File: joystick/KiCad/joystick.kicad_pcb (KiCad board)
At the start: 2 copper layers, 37 x 33 mm, 7 parts, among them J1 Conn_01x06_Pin, U1 COM-09032

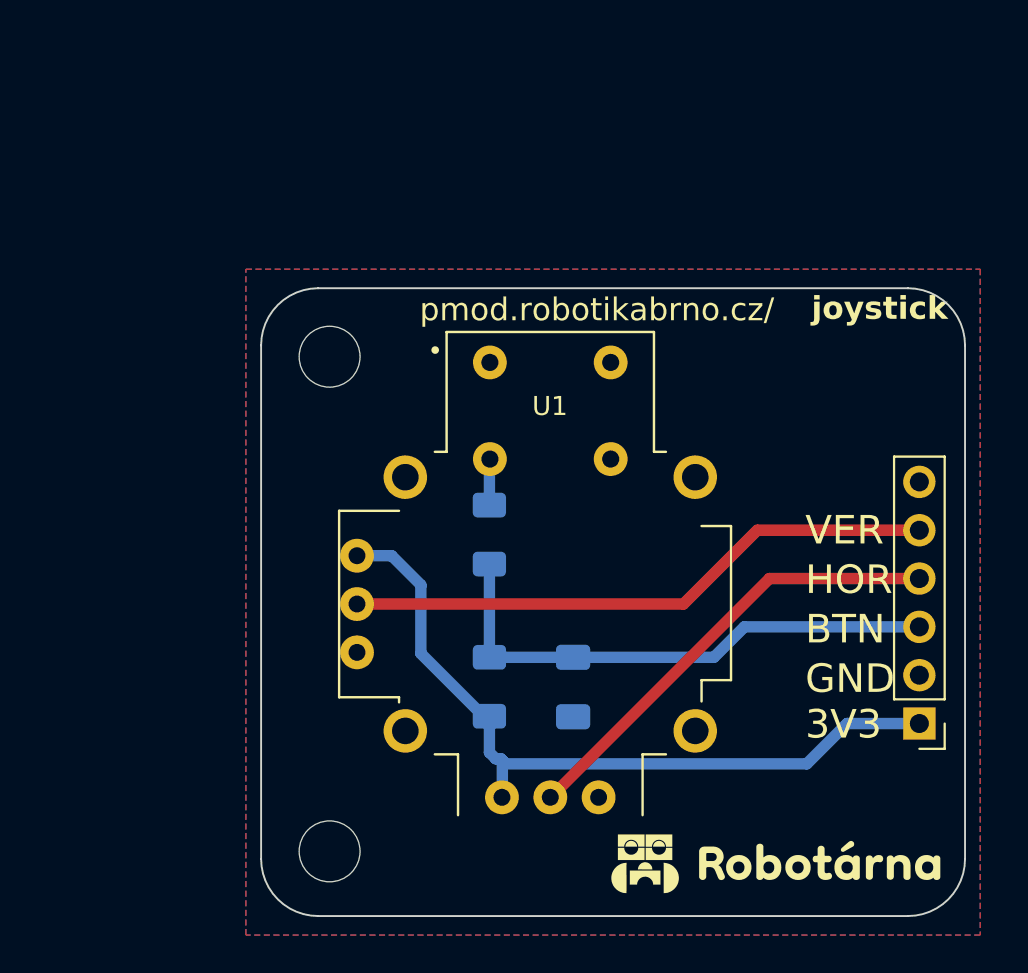
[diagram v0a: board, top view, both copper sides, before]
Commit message: Deployed d972a79 with MkDocs version: 1.6.0
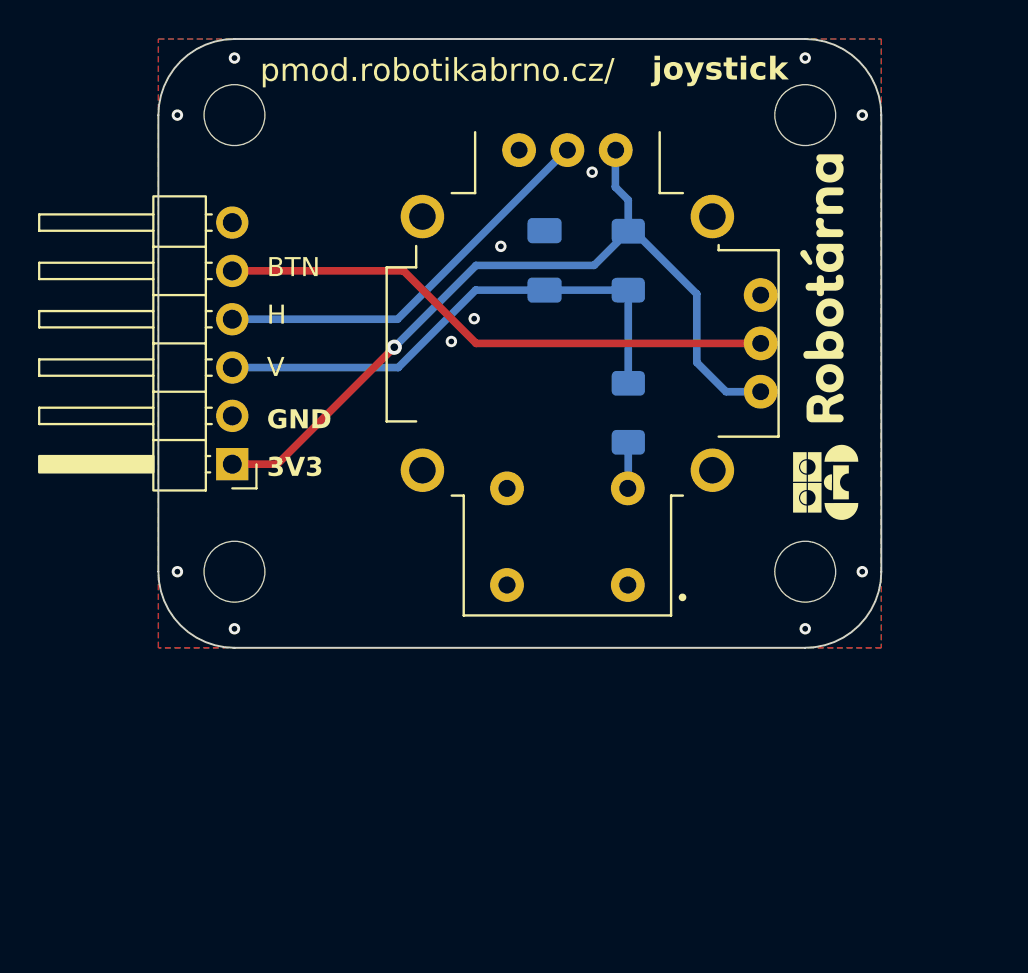
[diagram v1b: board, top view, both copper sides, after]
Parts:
- added H3: MountingHole, MountingHole:MountingHole_3.2mm_M3, F.Cu at (62.2, 48.7)
- added H4: MountingHole, MountingHole:MountingHole_3.2mm_M3, F.Cu at (62.2, 24.7)
- H1, H2: footprint MountingHole:MountingHole_3.2mm_M3_DIN965 -> MountingHole:MountingHole_3.2mm_M3
- J1: footprint Connector_PinHeader_2.54mm:PinHeader_1x06_P2.54mm_Vertical -> Connector_PinHeader_2.54mm:PinHeader_1x06_P2.54mm_Horizontal
- moved H2 46.1 mm to (92.2, 24.7), turned to 180 degrees
- moved J1 38.6 mm to (62.1, 43.0)
- moved H1 27.4 mm to (92.2, 48.7), turned to 180 degrees
- moved R1 23.6 mm to (82.9, 32.4), turned to 90 degrees
- moved C1 22.5 mm to (78.5, 32.3), turned to 90 degrees
- moved U1 13.7 mm to (79.7, 36.7), turned to 180 degrees
- moved R2 9.71 mm to (82.9, 40.4), turned to -90 degrees
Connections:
- C1 pad 1: /SEL -> /V
- J1 pad 3: /SEL -> /V
- J1 pad 5: /V -> /SEL
- R1 pad 1: /SEL -> /V
- R2 pad 1: /SEL -> /V
- U1 pad V2: /V -> /SEL
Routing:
- net /V: track 31.1 -> 27.4 mm
- net /H: track 24.1 -> 21.3 mm
- net /3V3: track 40.2 -> 43.0 mm, vias 0 -> 1
- net /SEL: track 28.2 -> 29.3 mm
- net /GND: vias 0 -> 12
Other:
- board size 37 x 33 mm -> 38 x 32 mm
- board text added: "32mm"
- board text added: "38mm"
- board text added: "H"
- board text added: "V"
- board text removed: "HOR"
- board text removed: "VER"
